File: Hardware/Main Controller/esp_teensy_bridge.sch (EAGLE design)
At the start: 47 parts, among them IC1 BQ79600PWRQ1, Q1 SI7611DN-T1-GE3, Q2 SI7611DN-T1-GE3, Q3 SI7611DN-T1-GE3, Q4 SI7611DN-T1-GE3

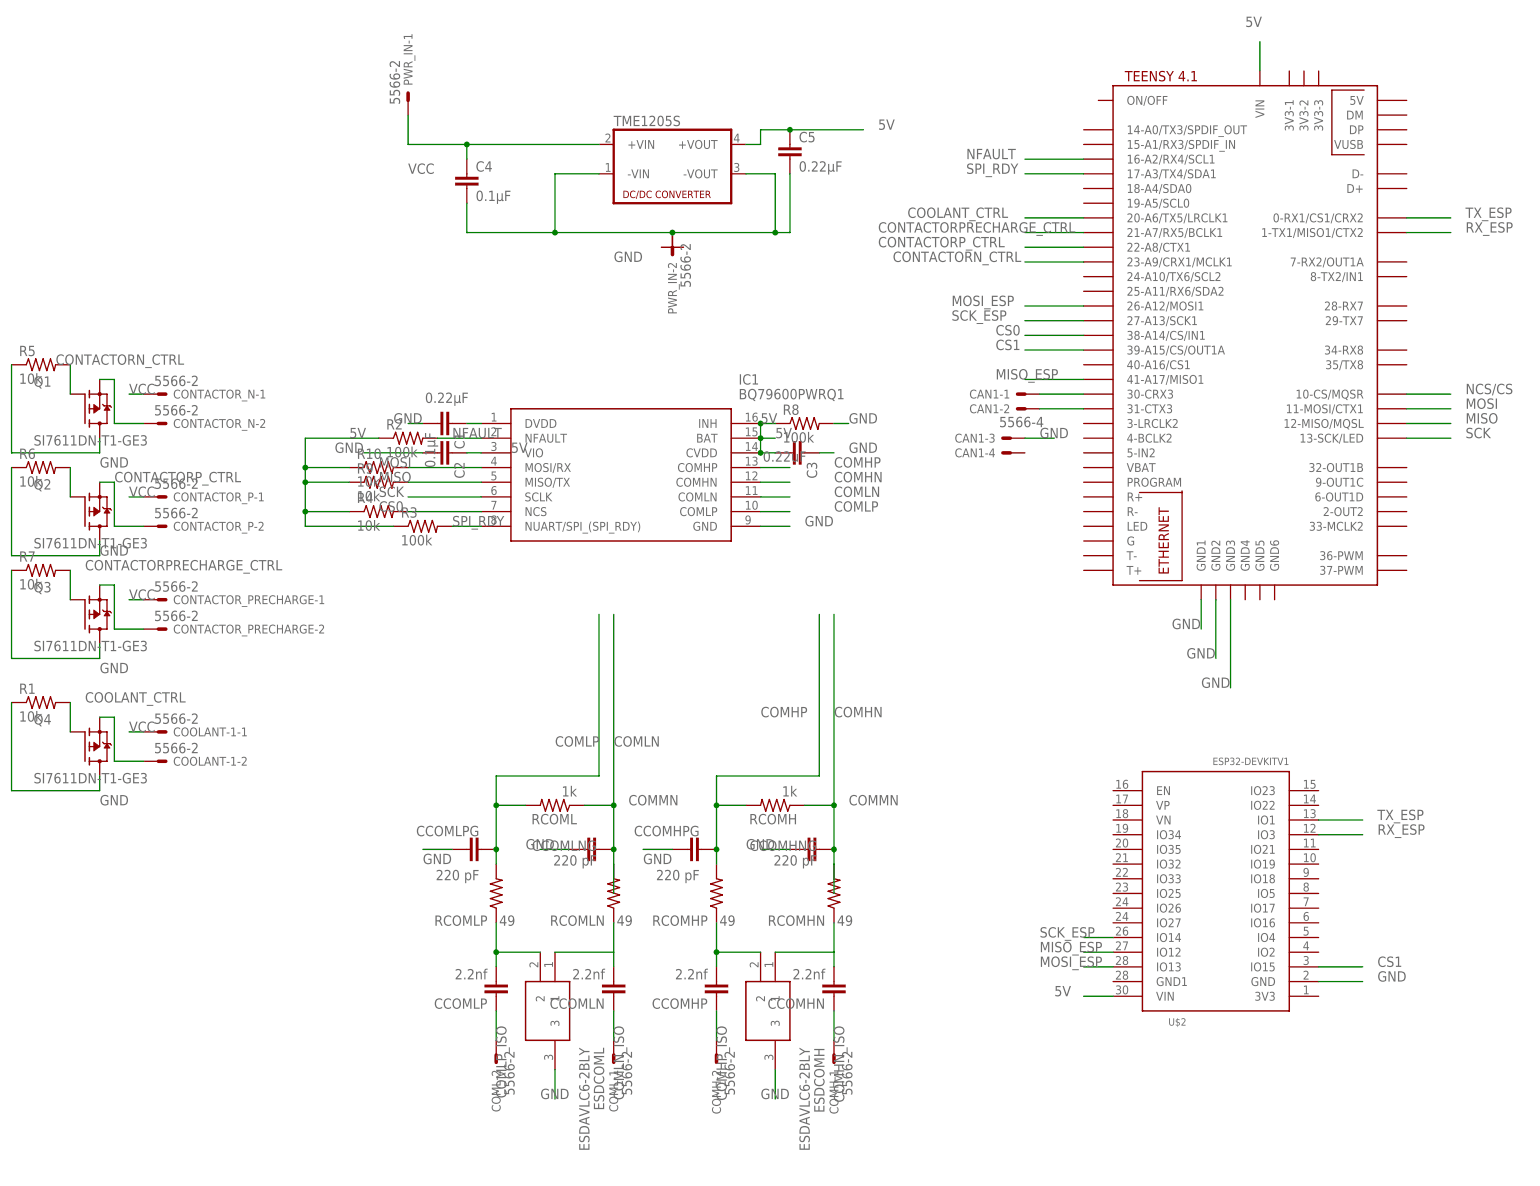
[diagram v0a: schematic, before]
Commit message: final additions hopefully
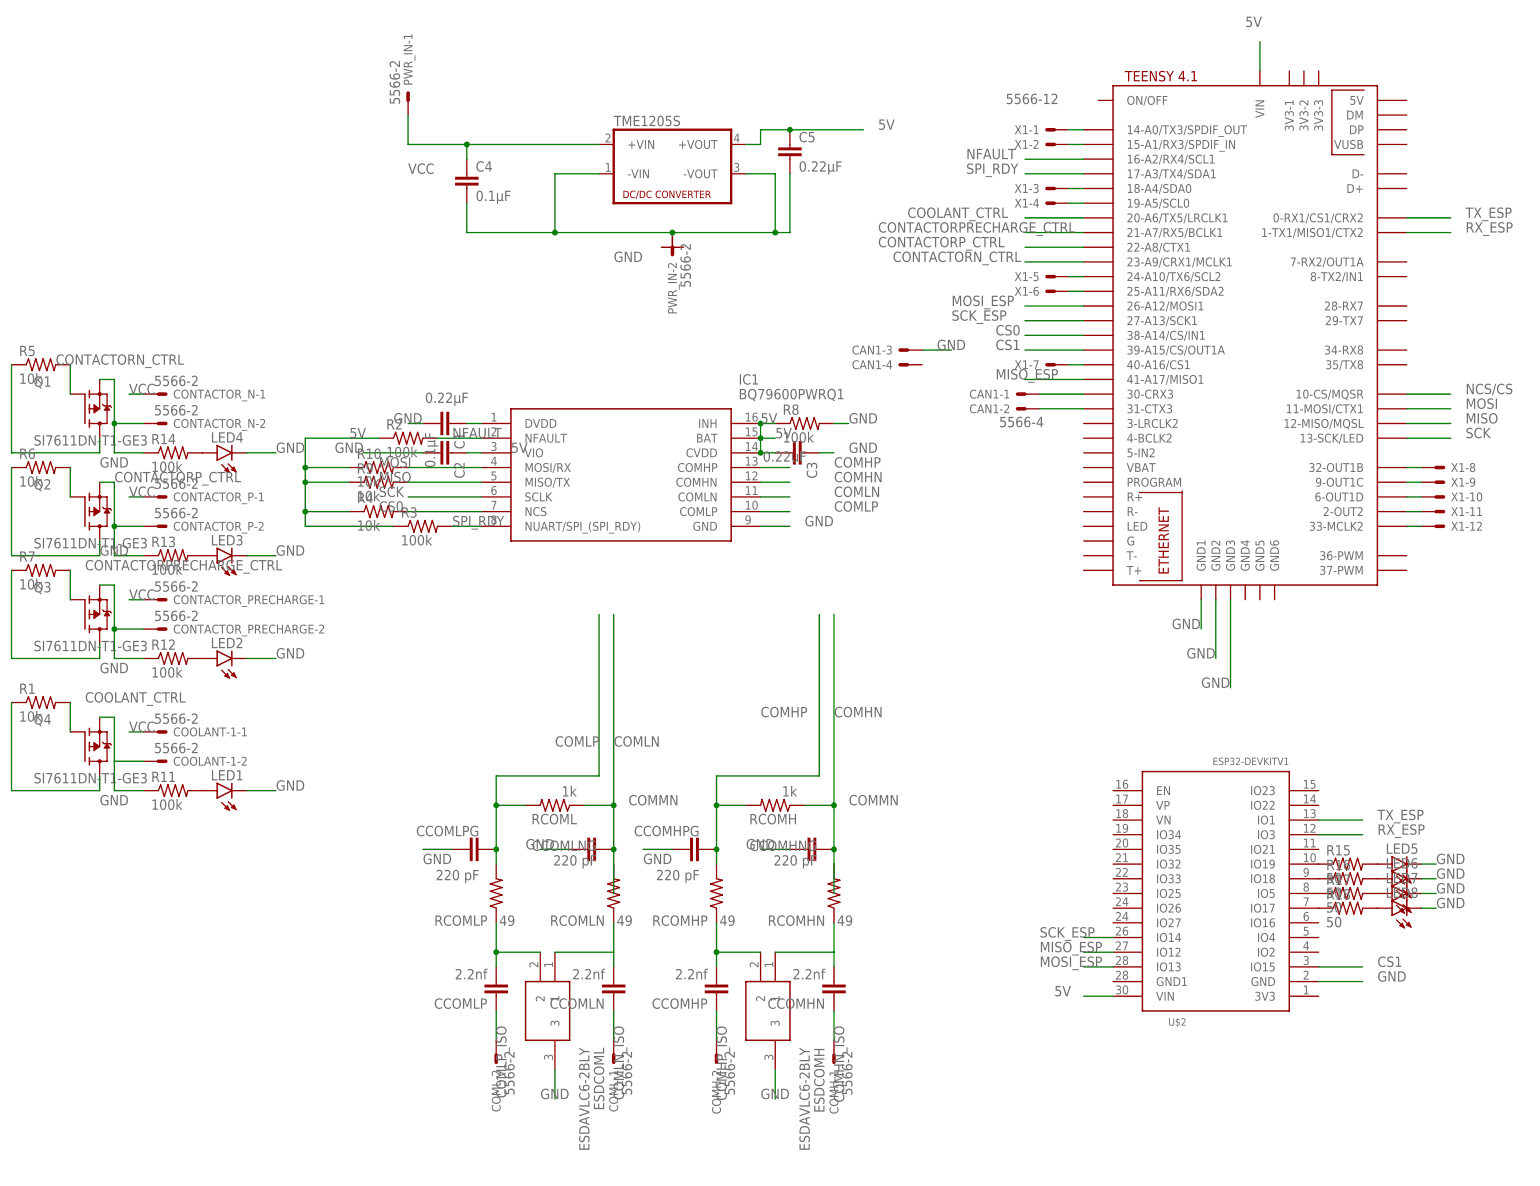
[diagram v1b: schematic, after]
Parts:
- added LED1, LED2, LED3, LED4, LED5, LED6, LED7, LED8: (no value), led:LEDSML0603
- added R11, R12, R13, R14: 100k, rcl:R-US_R0603
- added R15, R16, R17, R18: 50, rcl:R-US_R0603
- added X1: 5566-12, con-molex:5566-12
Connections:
- new net N$13: LED4.A, R14.2
- new net N$14: U$3.14-A0/TX3/SPDIF_OUT, X1-1.S
- new net N$17: U$3.15-A1/RX3/SPDIF_IN, X1-2.S
- new net N$18: U$3.18-A4/SDA0, X1-3.S
- new net N$19: U$3.19-A5/SCL0, X1-4.S
- new net N$20: U$3.24-A10/TX6/SCL2, X1-5.S
- new net N$21: U$3.25-A11/RX6/SDA2, X1-6.S
- new net N$22: U$3.40-A16/CS1, X1-7.S
- new net N$23: U$3.32-OUT1B, X1-8.S
- new net N$24: U$3.9-OUT1C, X1-9.S
- new net N$25: U$3.6-OUT1D, X1-10.S
- new net N$26: U$3.33-MCLK2, X1-12.S
- new net N$27: U$3.2-OUT2, X1-11.S
- new net N$28: R15.1, U$2.IO19
- new net N$29: R16.1, U$2.IO18
- new net N$3: LED1.A, R11.2
- new net N$30: R17.1, U$2.IO5
- new net N$31: R18.1, U$2.IO17
- new net N$32: LED5.A, R15.2
- new net N$33: LED6.A, R16.2
- new net N$34: LED7.A, R17.2
- new net N$35: LED8.A, R18.2
- new net N$4: LED2.A, R12.2
- new net N$9: LED3.A, R13.2
- net GND: now also LED1.C, LED2.C, LED3.C, LED4.C, LED5.C, LED6.C, LED7.C, LED8.C
- net N$12: now also R12.1
- net N$2: now also R13.1
- net N$5: now also R14.1
- net N$6: now also R11.1
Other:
- moved on the sheet: CAN1-3, CAN1-4
